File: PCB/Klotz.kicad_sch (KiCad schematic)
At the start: 55 parts, among them SW1 MX_SW_HS, SW10 MX_SW_HS, SW11 MX_SW_HS, SW12 MX_SW_HS, SW13 MX_SW_HS, SW14 MX_SW_HS, SW15 MX_SW_HS, SW16 MX_SW_HS, SW17 MX_SW_HS, SW18 RotaryEncoder, SW2 MX_SW_HS, SW3 MX_SW_HS, SW4 MX_SW_HS, SW5 MX_SW_HS, SW6 MX_SW_HS, SW7 MX_SW_HS, SW8 MX_SW_HS, SW9 MX_SW_HS, U1 nice!nano

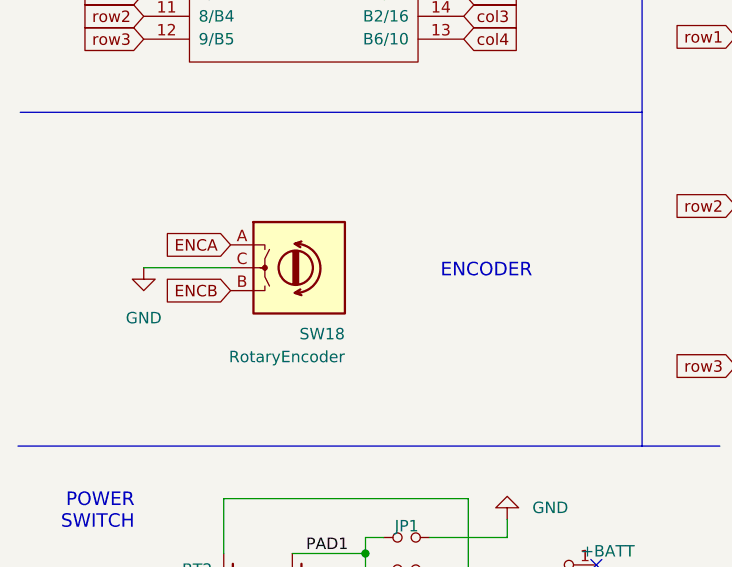
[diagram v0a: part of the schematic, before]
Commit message: init
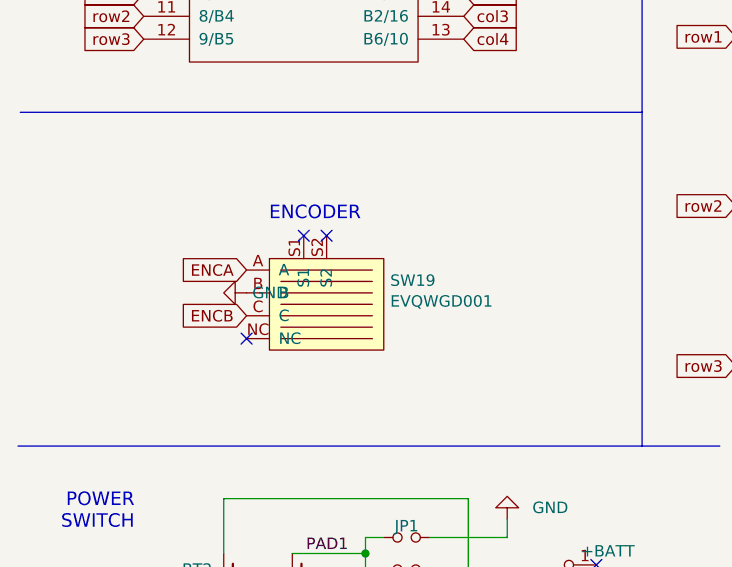
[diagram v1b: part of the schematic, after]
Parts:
- removed SW18: RotaryEncoder, Rotary_Encoder:RotaryEncoder_Alps_EC12E_Vertical_H20mm, symbol Device:RotaryEncoder
- added SW19: EVQWGD001, evq:EVQWGD001, symbol barobord:EVQWGD001
- RSW1: footprint (none) -> KLOTZ:ResetSW
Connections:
- net ENCA: now also SW19.A
- net ENCB: now also SW19.C
- net GND: now also SW19.B
- no-connect marks 5 -> 8
